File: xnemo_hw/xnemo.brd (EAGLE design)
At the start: 49.9 x 49 mm, 46 parts, among them J1 MICRO_USB_B_RECEPT, J2 DM3D_MICRO_SD, J3 HEADER_2X5_0.05_SMD, J4 HEADER_2X5_0.05_THRU, J5 HEADER_2X5_0.05_THRU, U1 LTC3559, U2 L3GD20, U3 STM32F405RG, U4 STM32F407VE, U5 HMC5883L, U6 ADXL345, U7 LSM303DLHC, U8 LSM303DLHC, X1 TXC_7A_XTAL

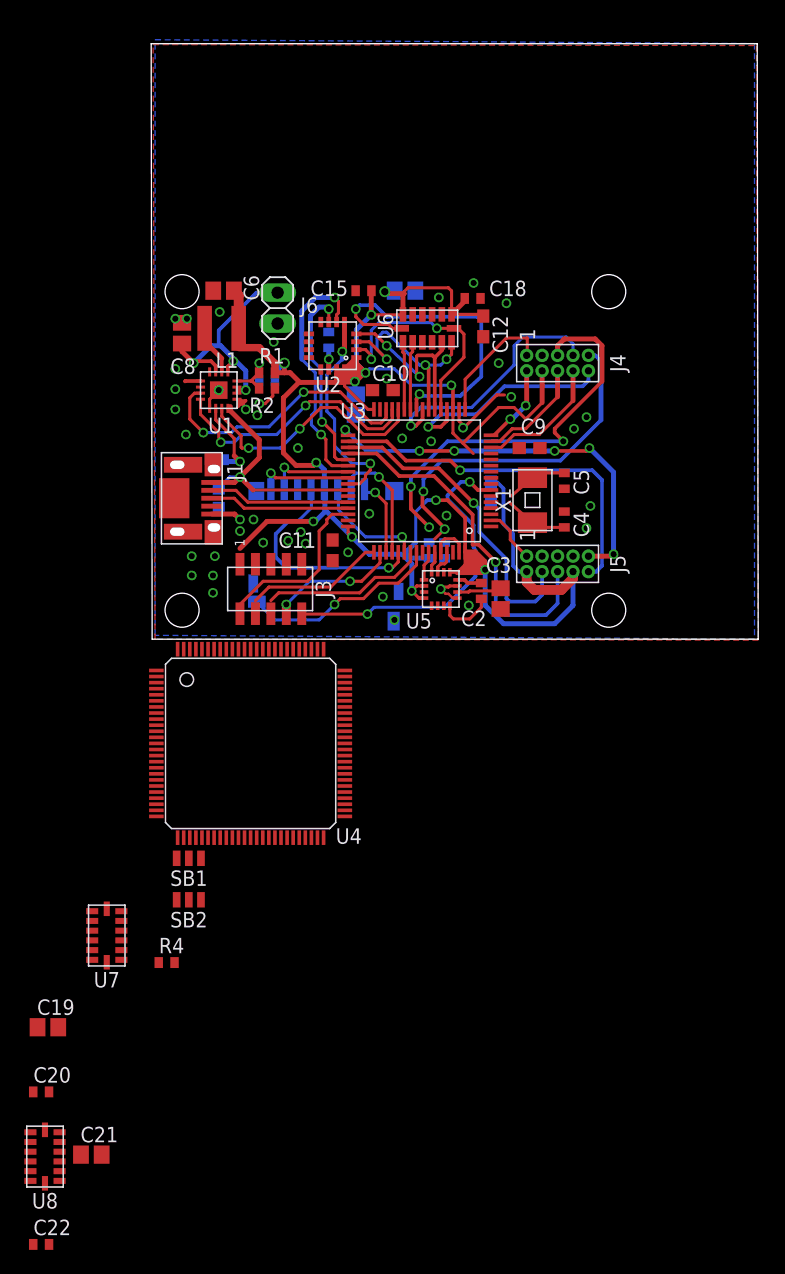
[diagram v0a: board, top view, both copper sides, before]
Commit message: Started routing
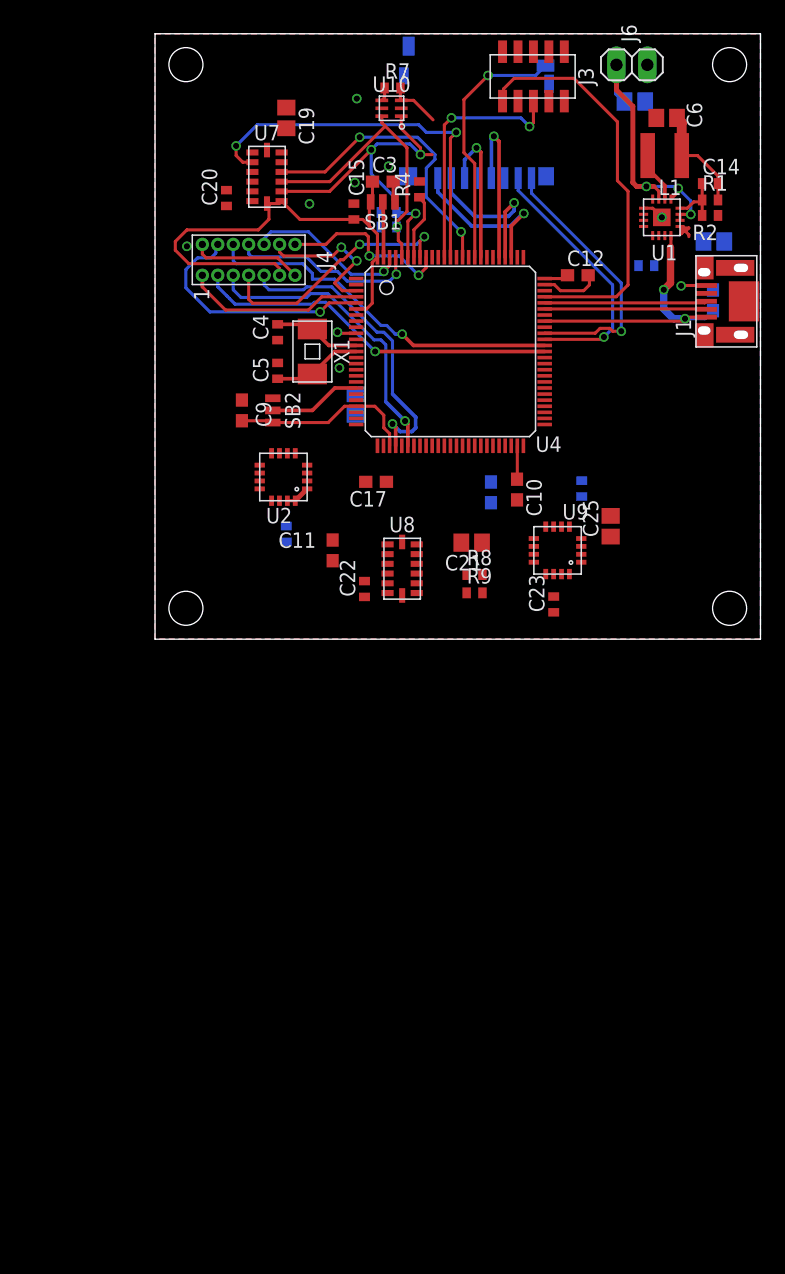
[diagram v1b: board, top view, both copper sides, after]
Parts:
- removed C18: 0.1u, resistor:C0402
- removed J5: HEADER_2X5_0.05_THRU, xnemo:HEADER_2X5_0.05_THRU
- removed U3: STM32F405RG, xnemo:ST_LQFP64
- removed U5: HMC5883L, xnemo:HW_LCC16_3X3
- removed U6: ADXL345, xnemo:AD_LGA14_3X5
- added C23: 10n, resistor:C0402
- added C24: 0.22u, resistor:C0402
- added C25: 10u, resistor:C0805
- added R7: 33k, resistor:R0402
- added R8, R9: 22k, resistor:R0402
- added U10: STTS751, xnemo:ST_UDFN-6L_2X2
- added U9: L3GD20, xnemo:ST_LGA16_4X4
- C17: value 10u -> 2.2u; device resistor:C0805 -> resistor:C0603
- C2: value 0.22u -> 10u; device resistor:C0402 -> resistor:C0805
- C3: value 4.7u -> 2.2u; device resistor:C0805 -> resistor:C0603
- J4: value HEADER_2X5_0.05_THRU -> HEADER_2X7; device xnemo:HEADER_2X5_0.05_THRU -> xnemo:HEADER_2X7_0.05X0.1_THRU
- moved C19 77.3 mm to (10.8, 42.9), turned to 270 degrees
- moved C20 75.1 mm to (5.87, 36.3), turned to 90 degrees
- moved R4 66.9 mm to (21.7, 37.0), turned to 90 degrees
- moved U7 63.8 mm to (9.21, 38.0), turned to 180 degrees
- moved C22 60.1 mm to (17.2, 4.13), turned to 90 degrees
- moved C21 59.2 mm to (26.0, 7.94), turned to 180 degrees
- moved U8 56.6 mm to (20.3, 5.79), turned to 180 degrees
- moved SB1 56.3 mm to (18.7, 36.0)
- moved J1 49.1 mm to (48.2, 27.8), turned to 90 degrees
- moved J3 47.4 mm to (31.1, 46.3)
- moved C7 43.8 mm to (45.9, 27.9), turned to 270 degrees
- moved C8 41.8 mm to (39.4, 44.2), flipped to the bottom, turned to 0 degrees
- moved SB2 40.8 mm to (9.68, 18.8), turned to 90 degrees
- moved J2 40.0 mm to (27.1, 43.9), turned to 0 degrees
- moved C14 39.9 mm to (45.6, 37.5), flipped to the top, turned to 0 degrees
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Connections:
- net GYR_RES renamed GYR_RES1
- net N$21 renamed SPI2_NSS_WS
- net N$28 renamed COMP2_C1
- net N$52 renamed COMP1_C1
- net SPI2_MISO renamed SPI2_MISO_EXT_SD
- net SPI2_MOSI renamed SPI2_MOSI_SD
- net SPI2_SCK renamed SPI2_SCK_CK
- removed net ACC_INT1: U3.P$27, U6.P$8
- removed net ACC_INT2: U3.P$26, U6.P$9
- removed net DCMI_D0: U4.P$63
- removed net GYR_DRDY: U2.P$6, U3.P$38
- removed net GYR_INT1: U2.P$7, U3.P$37
- removed net I2C_SCL: J4.P$5, U5.P$1
- removed net I2C_SDA: J4.P$9, U5.P$16
- removed net JTCK: U3.P$49
- removed net JTDI: U3.P$50
- removed net JTDO: U3.P$55
- removed net JTMS: U3.P$46
- removed net MAG_C1: C3.1, U5.P$10
- removed net MAG_DRDY: U3.P$61, U5.P$15
- removed net MAG_SETC: C2.2, U5.P$12
- removed net MAG_SETP: C2.1, U5.P$8
- removed net N$24: U4.P$75
- removed net N$30: U4.P$81
- removed net N$31: U4.P$82
- removed net N$33: U4.P$84
- removed net N$34: U4.P$85
- removed net N$35: U4.P$86
- removed net N$36: U4.P$87
- removed net N$37: U4.P$88
- removed net N$59: U4.P$16
- removed net N$60: U4.P$17
- removed net N$61: U4.P$18
- removed net N$63: U4.P$20
- removed net N$70: U4.P$27
- removed net N$71: U4.P$28
- removed net N$84: U4.P$41
- removed net N$85: U4.P$42
- removed net N$86: U4.P$43
- removed net N$87: U4.P$44
- removed net N$88: U4.P$45
- removed net N$89: U4.P$46
- removed net N$9: U4.P$64
- removed net N$93: U4.P$50
- removed net PA0: J4.P$8, U3.P$14
- removed net PA1: J4.P$6, U3.P$15
- removed net PA10: U3.P$43
- removed net PA2: J4.P$2, U3.P$16
- removed net PA3: J4.P$1, U3.P$17
- removed net PA4: J4.P$10, U3.P$20
- removed net PB12: J5.P$9, U3.P$33
- removed net PB13: J5.P$10, U3.P$34
- removed net PB14: J5.P$4, U3.P$35
- removed net PB15: J5.P$6, U3.P$36
- removed net PC0: U3.P$8
- removed net PC1: U3.P$9
- removed net PC13: J5.P$1, U3.P$2
- removed net PC2: U3.P$10
- removed net PC3: U3.P$11
- removed net PC4: J4.P$7, U3.P$24
- removed net RESET: U3.P$7
- removed net SPI_CLK: U2.P$2, U3.P$21, U6.P$14
- removed net SPI_CS_ACC: U3.P$25, U6.P$7
- removed net SPI_CS_GYR: U2.P$5, U3.P$41
- removed net SPI_MISO: U2.P$4, U3.P$22, U6.P$12
- removed net SPI_MOSI: U2.P$3, U3.P$23, U6.P$13
- new net DCMI_D0_MCK: J4.P$4, U4.P$63
- new net DCMI_D1: J4.P$6, U4.P$64
- new net GYR1_DRDY: U2.P$6, U4.P$17
- new net GYR1_INT1: U2.P$7, U4.P$18
- new net GYR2_DRDY: U4.P$45, U9.P$6
- new net GYR2_INT1: U4.P$44, U9.P$7
- new net GYR_RES2: C23.2, U9.P$14
- new net SPI_CS_GYR1: U2.P$5, U4.P$16
- new net SPI_CS_GYR2: U4.P$46, U9.P$5
- new net TEMP1_ADDR: R7.1, U10.P$4
- new net TEMP1_EVT: U10.P$2
- net 3V3: now also C17.2, C2.1, C24.2, C25.1, C3.1, J4.P$11, R7.2, R8.2, R9.2, U10.P$3, U4.P$28, U4.P$50, U4.P$75, U9.P$1, U9.P$15, U9.P$16; no longer C17.1, C18.2, J4.P$4, J5.P$2, J5.P$8, U3.P$19, U3.P$32, U3.P$48, U3.P$64, U5.P$13, U5.P$2, U5.P$4, U6.P$1, U6.P$6
- net COMP1_DRDY: now also U4.P$88
- net COMP1_INT1: now also U4.P$86
- net COMP1_INT2: now also U4.P$87
- net COMP2_DRDY: now also U4.P$41
- net COMP2_INT1: now also U4.P$43
- net COMP2_INT2: now also U4.P$42
- net DCMI_D2: now also J4.P$8
- net DCMI_D3: now also J4.P$10
- net DCMI_D4: now also J4.P$12
- net DCMI_D5: now also J4.P$14
- net DCMI_D6: now also J4.P$1
- net DCMI_D7: now also J4.P$3
- net DCMI_HSYNC: now also J4.P$9
- net DCMI_PIXCLK: now also J4.P$5
- net DCMI_VSYNC: now also J4.P$7
- net GND: now also C17.1, C2.2, C23.1, C24.1, C25.2, J4.P$13, J4.P$2, U10.P$5, U4.P$20, U4.P$27, U9.P$10, U9.P$11, U9.P$12, U9.P$13, U9.P$8, U9.P$9; no longer C17.2, C18.1, J4.P$3, J5.P$3, J5.P$5, J5.P$7, U3.P$18, U3.P$60, U3.P$63, U5.P$11, U5.P$9, U6.P$2, U6.P$4, U6.P$5
- net I2C1_SCL: now also U10.P$1
- net I2C1_SDA: now also U10.P$6
- net I2C2_SCL: now also R9.1
- net I2C2_SDA: now also R8.1
- net POW_CHRG: now also U4.P$81; no longer U3.P$28
- net POW_HPWR: now also U4.P$82; no longer U3.P$29
- net POW_SUSP: now also U4.P$85; no longer U3.P$30
- net SD_CLK: no longer U3.P$53
- net SD_CMD: no longer U3.P$54
- net SD_DAT0_I2C3_SCL: no longer U3.P$39
- net SD_DAT1_I2C3_SDA: no longer U3.P$40
- net SD_DAT2: no longer U3.P$51
- net SD_DAT3: no longer U3.P$52
- net SD_DET: now also U4.P$84; no longer U3.P$56
- net SPI1_MISO: now also U2.P$4, U9.P$4
- net SPI1_MOSI: now also U2.P$3, U9.P$3
- net SPI1_SCK: now also U2.P$2, U9.P$2
- net USB_D+: no longer U3.P$45
- net USB_D-: no longer U3.P$44
- net VUSB: no longer U3.P$42
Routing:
- net 3V3: track 182.2 -> 74.3 mm, vias 12 -> 0
- net I2C_SCL: track 34.9 -> 0.00 mm, vias 3 -> 0
- net SWDIO: track 0.00 -> 33.2 mm
- net PB12: track 33.1 -> 0.00 mm, vias 6 -> 0
- net COMP1_DRDY: track 0.00 -> 31.9 mm, vias 0 -> 2
- net PB13: track 30.6 -> 0.00 mm, vias 1 -> 0
- net I2C_SDA: track 30.5 -> 0.00 mm, vias 2 -> 0
- net DCMI_D0_MCK: track 0.00 -> 30.2 mm, vias 0 -> 1
- net DCMI_D1: track 0.00 -> 30.1 mm, vias 0 -> 1
- net I2C1_SCL: track 0.00 -> 29.9 mm, vias 0 -> 3
- net PB15: track 29.3 -> 0.00 mm, vias 1 -> 0
- net SPI_CS_ACC: track 27.5 -> 0.00 mm, vias 2 -> 0
- net RESET: track 27.2 -> 0.00 mm, vias 2 -> 0
- net PB14: track 26.4 -> 0.00 mm, vias 1 -> 0
- net DCMI_HSYNC: track 0.00 -> 25.6 mm, vias 0 -> 1
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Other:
- board size 49.9 x 49 mm -> 49.8 x 49.8 mm
- board text removed: "bnahill@gmail.com"
- board text removed: "xNEMO r1"
